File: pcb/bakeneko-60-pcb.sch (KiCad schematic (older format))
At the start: 18 parts, among them J1 JST SH 4-pin, J2 AVR-ISP-6, SW1 Reset, U1 SRV05-4, U2 ATmega32U4-AU, Y1 16MHz

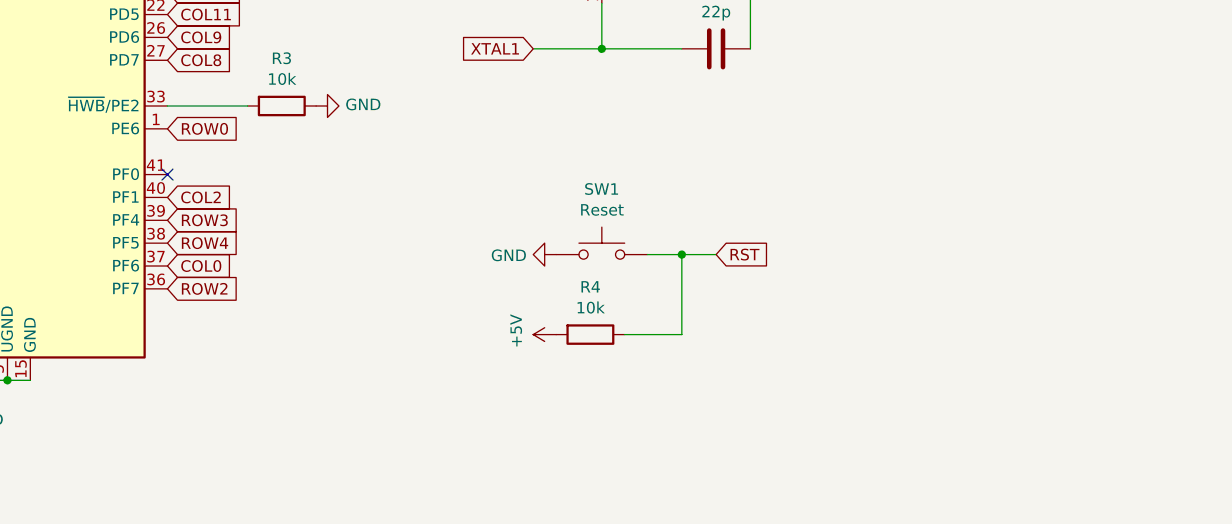
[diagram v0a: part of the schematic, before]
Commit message: Bakeneko-70 intial implementation
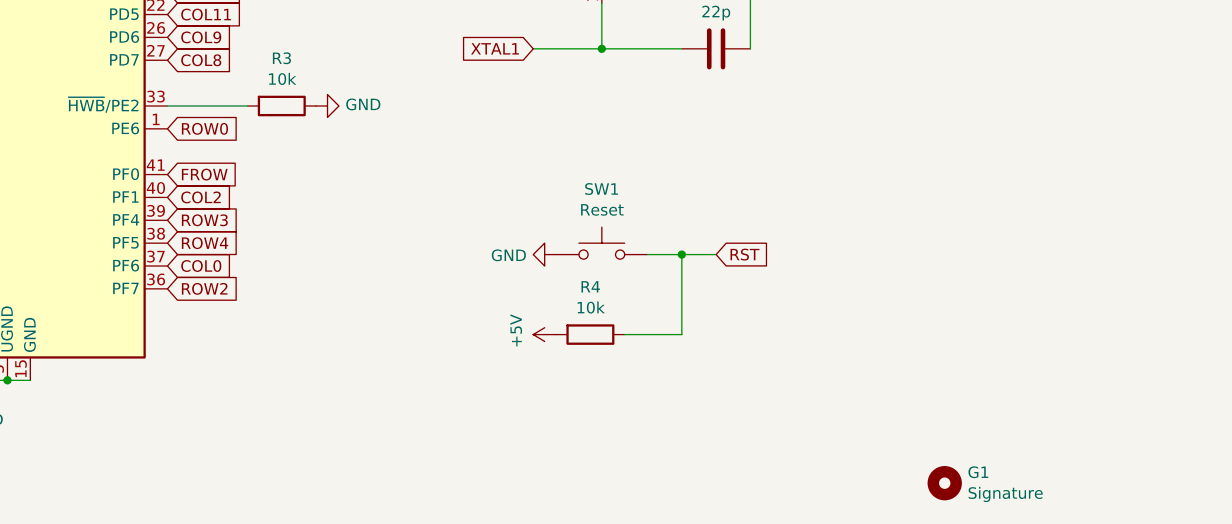
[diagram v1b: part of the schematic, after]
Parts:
- added G1: Signature, Ramon:Signature, symbol Mechanical:MountingHole
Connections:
- net FROW: now reaches U2.41 (PF0)
- no-connect marks 5 -> 4
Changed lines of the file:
@@
 Text GLabel 2950 4900 2    50   Input ~ 0
 COL3
-NoConn ~ 2950 6300
 $Comp
 L power:GND #PWR07
@@
 NoConn ~ 6850 1500
 NoConn ~ 5850 1700
+Text GLabel 2950 6300 2    50   Input ~ 0
+FROW
+$Comp
+L Mechanical:MountingHole G1
+U 1 1 619548B4
+P 6350 7650
+F 0 "G1" H 6450 7696 50  0000 L CNN
+F 1 "Signature" H 6450 7605 50  0000 L CNN
+F 2 "Ramon:Signature" H 6350 7650 50  0001 C CNN
+F 3 "~" H 6350 7650 50  0001 C CNN
+	1    6350 7650
+	1    0    0    -1
+$EndComp
 $EndSCHEMATC
